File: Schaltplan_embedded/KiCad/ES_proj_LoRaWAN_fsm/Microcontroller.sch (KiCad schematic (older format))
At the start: 15 parts, among them J1 Conn_02x05_Odd_Even, U1 STM32L476RGTx, Y1 Crystal

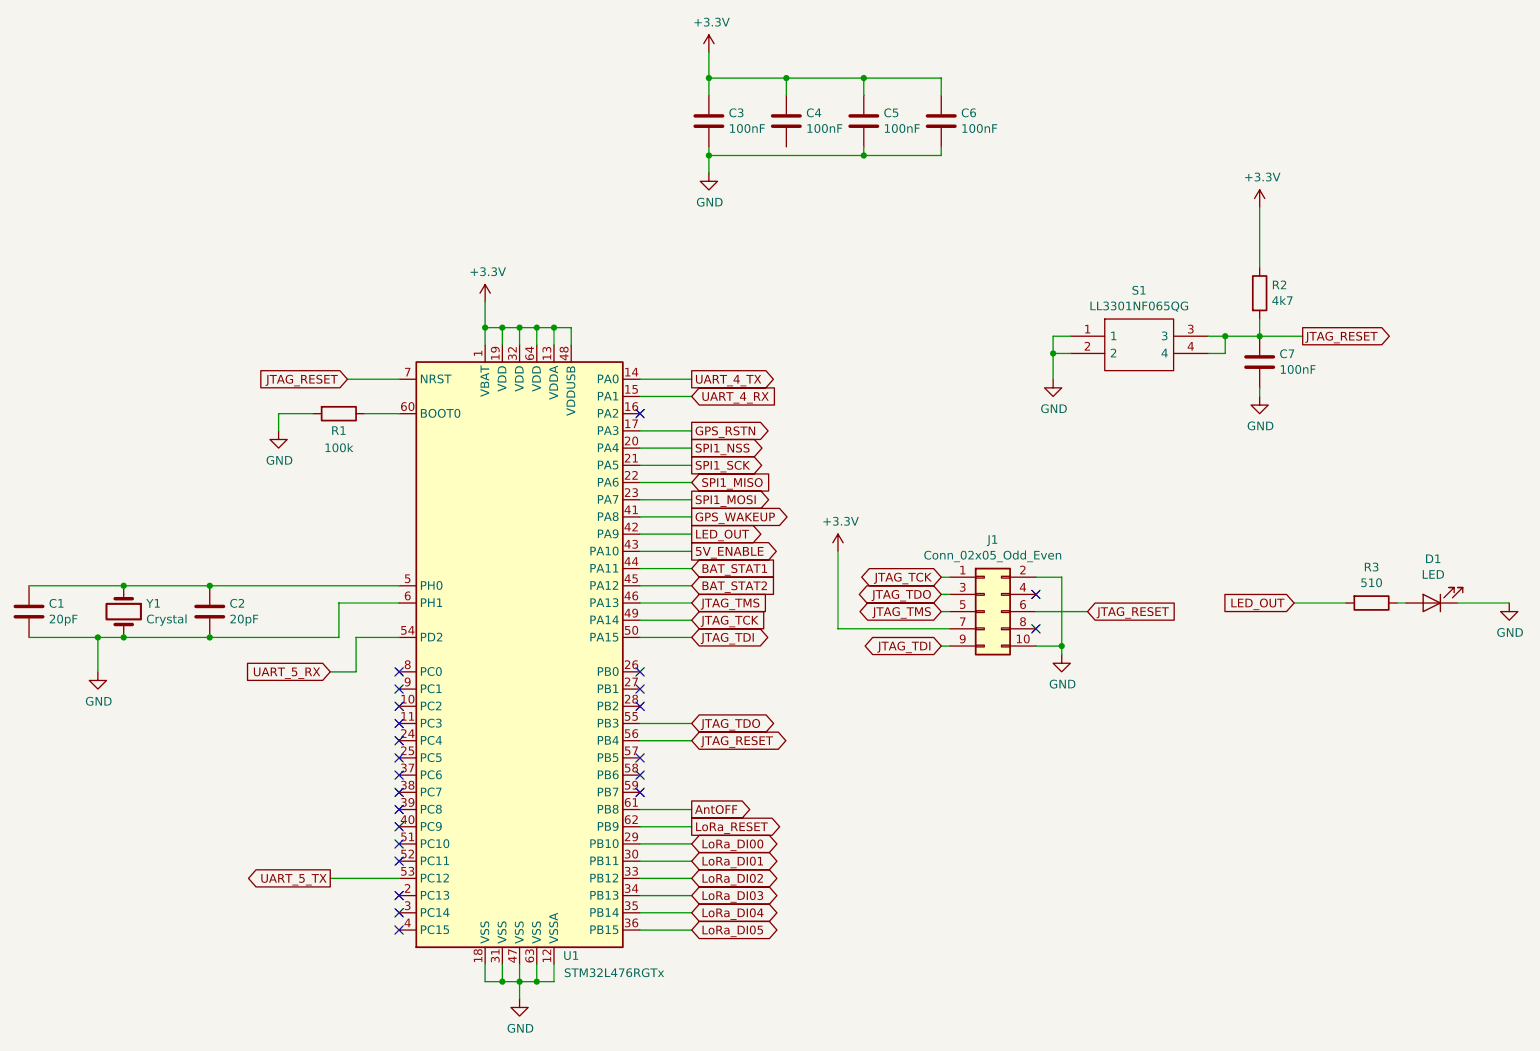
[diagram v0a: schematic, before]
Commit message: no message
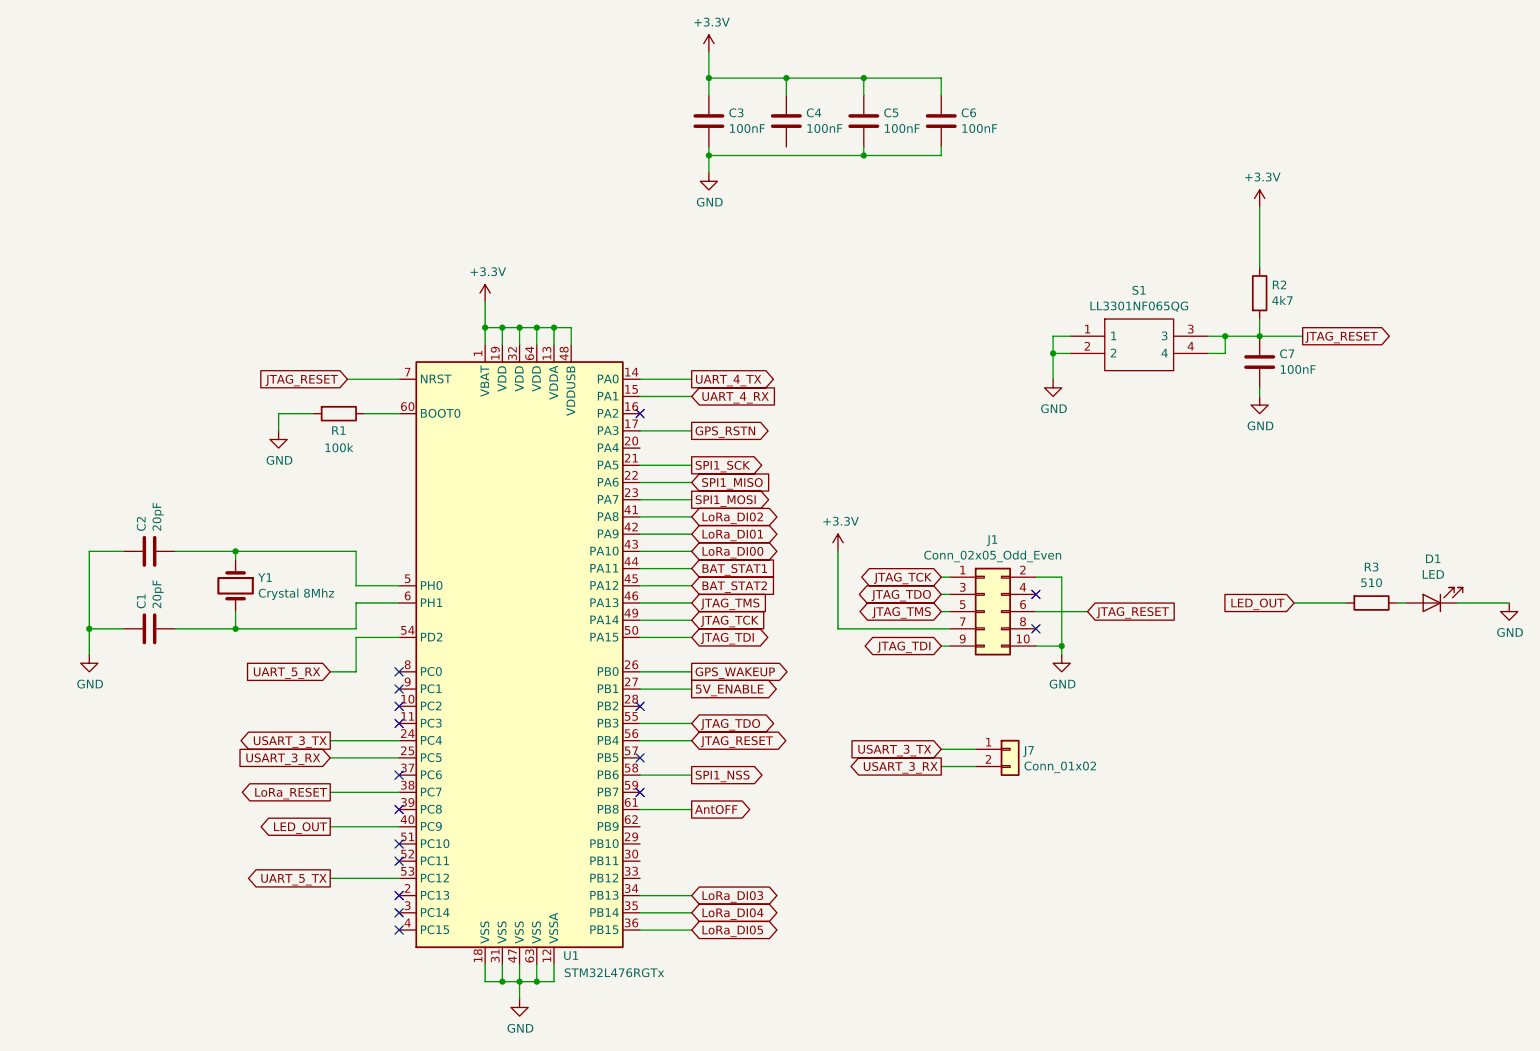
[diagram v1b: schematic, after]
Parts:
- added J7: Conn_01x02, Pin_Headers:Pin_Header_Straight_1x02_Pitch1.00mm, symbol Connector_Generic:Conn_01x02
- Y1: value Crystal -> Crystal 8Mhz; footprint SamacSys_Parts:ABS2532768KHZT -> Crystals:Crystal_SMD_HC49-SD_HandSoldering
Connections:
- net 5V_ENABLE: now also U1.27 (PB1); no longer U1.43 (PA10)
- net GND: now also C1.1, C2.1; no longer C1.2, C2.2, U1.6 (PH1), Y1.2
- net GPS_WAKEUP: now also U1.26 (PB0); no longer U1.41 (PA8)
- net LED_OUT: now also U1.40 (PC9); no longer U1.42 (PA9)
- net LoRa_DI00: now also U1.43 (PA10); no longer U1.29 (PB10)
- net LoRa_DI01: now also U1.42 (PA9); no longer U1.30 (PB11)
- net LoRa_DI02: now also U1.41 (PA8); no longer U1.33 (PB12)
- net LoRa_RESET: now also U1.38 (PC7); no longer U1.62 (PB9)
- net SPI1_NSS: now also U1.58 (PB6); no longer U1.20 (PA4)
- net USART_3_TX: now reaches U1.24 (PC4)
- net USART_3_TX: now also J7.1 (Pin_1)
- net USART_3_RX: now reaches U1.25 (PC5)
- net USART_3_RX: now also J7.2 (Pin_2)
- net at U1.5 (PH0), Y1.1: now also C2.2; no longer C1.1, C2.1
- new net: C1.2, U1.6 (PH1), Y1.2
- no-connect marks 24 -> 17
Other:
- moved on the sheet: C1, C2, Y1
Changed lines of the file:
@@
 L power:GND #PWR0101
 U 1 1 5DC1A6C7
-P 1650 4750
-F 0 "#PWR0101" H 1650 4500 50  0001 C CNN
-F 1 "GND" H 1655 4577 50  0000 C CNN
-F 2 "" H 1650 4750 50  0001 C CNN
-F 3 "" H 1650 4750 50  0001 C CNN
-	1    1650 4750
+P 1600 4650
+F 0 "#PWR0101" H 1600 4400 50  0001 C CNN
+F 1 "GND" H 1605 4477 50  0000 C CNN
+F 2 "" H 1600 4650 50  0001 C CNN
+F 3 "" H 1600 4650 50  0001 C CNN
+	1    1600 4650
 	1    0    0    -1
 $EndComp
@@
 L Device:Crystal Y1
 U 1 1 5DC1A7A3
-P 1800 4400
-F 0 "Y1" V 1754 4531 50  0000 L CNN
-F 1 "Crystal" V 1845 4531 50  0000 L CNN
-F 2 "SamacSys_Parts:ABS2532768KHZT" H 1800 4400 50  0001 C CNN
-F 3 "~" H 1800 4400 50  0001 C CNN
-	1    1800 4400
+P 2450 4250
+F 0 "Y1" V 2404 4381 50  0000 L CNN
+F 1 "Crystal 8Mhz" V 2495 4381 50  0000 L CNN
+F 2 "Crystals:Crystal_SMD_HC49-SD_HandSoldering" H 2450 4250 50  0001 C CNN
+F 3 "~" H 2450 4250 50  0001 C CNN
+	1    2450 4250
 	0    1    1    0
 $EndComp
@@
 L Device:C C1
 U 1 1 5DC1A815
-P 1250 4400
-F 0 "C1" H 1365 4446 50  0000 L CNN
-F 1 "20pF" H 1365 4355 50  0000 L CNN
-F 2 "Capacitors_SMD:C_0603_HandSoldering" H 1288 4250 50  0001 C CNN
-F 3 "~" H 1250 4400 50  0001 C CNN
-	1    1250 4400
-	1    0    0    -1
-$EndComp
-$Comp
-L Device:C C2
-U 1 1 5DC1A899
-P 2300 4400
-F 0 "C2" H 2415 4446 50  0000 L CNN
-F 1 "20pF" H 2415 4355 50  0000 L CNN
-F 2 "Capacitors_SMD:C_0603_HandSoldering" H 2338 4250 50  0001 C CNN
-F 3 "~" H 2300 4400 50  0001 C CNN
-	1    2300 4400
-	1    0    0    -1
-$EndComp
-Wire Wire Line
-	1250 4550 1650 4550
-Wire Wire Line
-	2300 4550 1800 4550
-Connection ~ 1800 4550
-Wire Wire Line
-	1650 4750 1650 4550
-Connection ~ 1650 4550
-Wire Wire Line
-	1650 4550 1800 4550
-Wire Wire Line
-	1250 4250 1800 4250
-Wire Wire Line
-	2300 4250 1800 4250
-Connection ~ 1800 4250
-Connection ~ 2300 4250
-Connection ~ 2300 4550
-Wire Wire Line
-	2300 4550 3050 4550
-Wire Wire Line
-	2300 4250 3400 4250
-Wire Wire Line
-	3050 4550 3050 4350
-Wire Wire Line
-	3050 4350 3400 4350
+P 1950 4500
+F 0 "C1" H 2065 4546 50  0000 L CNN
+F 1 "20pF" H 2065 4455 50  0000 L CNN
+F 2 "Capacitors_SMD:C_0603_HandSoldering" H 1988 4350 50  0001 C CNN
+F 3 "~" H 1950 4500 50  0001 C CNN
+	1    1950 4500
+	0    -1   -1   0
+$EndComp
 $Comp
 L power:GND #PWR0102
@@
 Wire Wire Line
 	6550 1300 6550 1400
-Text GLabel 5100 3450 2    50   Output ~ 0
+Text GLabel 5100 5350 2    50   Output ~ 0
 SPI1_NSS
-Wire Wire Line
-	4800 3450 5100 3450
 Text GLabel 5100 3550 2    50   Output ~ 0
 SPI1_SCK
@@
 Wire Wire Line
 	4800 3650 5100 3650
-Wire Wire Line
-	4800 3750 5100 3750
 Text GLabel 5100 3150 2    50   Input ~ 0
 UART_4_RX
@@
 Wire Wire Line
 	2700 3250 2700 3350
-Text GLabel 5100 3950 2    50   Output ~ 0
+Text GLabel 3000 5650 0    50   Output ~ 0
 LED_OUT
-Wire Wire Line
-	5100 3950 4800 3950
 Text GLabel 8600 4350 0    50   Input ~ 0
 LED_OUT
@@
 Wire Wire Line
 	9550 4350 9850 4350
-Text GLabel 5100 4050 2    51   Output ~ 0
+Text GLabel 5100 4850 2    51   Output ~ 0
 5V_ENABLE
 NoConn ~ 4800 5450
-NoConn ~ 4800 5350
 NoConn ~ 4800 5250
 NoConn ~ 3400 6250
@@
 NoConn ~ 3400 5850
 NoConn ~ 3400 5750
-NoConn ~ 3400 5650
 NoConn ~ 3400 5550
-NoConn ~ 3400 5450
 NoConn ~ 3400 5350
-NoConn ~ 3400 5250
-NoConn ~ 3400 5150
 NoConn ~ 3400 5050
 NoConn ~ 3400 4950
@@
 NoConn ~ 3400 4750
 NoConn ~ 4800 4950
-NoConn ~ 4800 4850
-NoConn ~ 4800 4750
 NoConn ~ 4800 3250
 Text GLabel 3100 3050 0    50   Input ~ 0
@@
 Wire Wire Line
 	4800 4250 5100 4250
-Text GLabel 5100 3850 2    50   Output ~ 0
+Text GLabel 5100 4750 2    50   Output ~ 0
 GPS_WAKEUP
 Text GLabel 5100 3350 2    50   Output ~ 0
@@
 Wire Wire Line
 	4800 3350 5100 3350
-Text GLabel 5100 5850 2    50   BiDi ~ 0
+Text GLabel 5100 3950 2    50   BiDi ~ 0
 LoRa_DI01
-Text GLabel 5100 5750 2    50   BiDi ~ 0
+Text GLabel 5100 4050 2    50   BiDi ~ 0
 LoRa_DI00
-Text GLabel 5100 5950 2    50   BiDi ~ 0
+Text GLabel 5100 3850 2    50   BiDi ~ 0
 LoRa_DI02
 Text GLabel 5100 6050 2    50   BiDi ~ 0
@@
 LoRa_DI05
 Wire Wire Line
-	4800 5750 5100 5750
-Wire Wire Line
-	4800 5850 5100 5850
-Wire Wire Line
-	4800 5950 5100 5950
-Wire Wire Line
 	4800 6050 5100 6050
 Wire Wire Line
@@
 Wire Wire Line
 	4800 6250 5100 6250
-Text GLabel 5100 5650 2    50   Output ~ 0
+Text GLabel 3000 5450 0    50   Output ~ 0
 LoRa_RESET
-Wire Wire Line
-	4800 5650 5100 5650
-$Comp
-L MCU_ST_STM32L4:STM32L476RGTx U1
-U 1 1 5DC1A60F
-P 4100 4650
-F 0 "U1" H 4400 2900 50  0000 C CNN
-F 1 "STM32L476RGTx" H 4650 2800 50  0000 C CNN
-F 2 "Housings_QFP:LQFP-64_10x10mm_Pitch0.5mm" H 3500 2950 50  0001 R CNN
-F 3 "http://www.st.com/st-web-ui/static/active/en/resource/technical/document/datasheet/DM00108832.pdf" H 4100 4650 50  0001 C CNN
-	1    4100 4650
-	1    0    0    -1
-$EndComp
 Wire Wire Line
 	3900 6450 3900 6550
@@
 Wire Wire Line
 	4800 5550 5100 5550
-Wire Wire Line
-	4800 4050 5100 4050
-Wire Wire Line
-	4800 3850 5100 3850
 $Comp
 L power:+3.3V #PWR0114
@@
 Wire Wire Line
 	8200 2800 8400 2800
+Wire Wire Line
+	4800 3750 5100 3750
+Wire Wire Line
+	4800 5350 5100 5350
+Wire Wire Line
+	4800 4050 5100 4050
+Wire Wire Line
+	4800 3950 5100 3950
+Wire Wire Line
+	4800 3850 5100 3850
+Wire Wire Line
+	3000 5650 3400 5650
+$Comp
+L MCU_ST_STM32L4:STM32L476RGTx U1
+U 1 1 5DC1A60F
+P 4100 4650
+F 0 "U1" H 4400 2900 50  0000 C CNN
+F 1 "STM32L476RGTx" H 4650 2800 50  0000 C CNN
+F 2 "Housings_QFP:LQFP-64_10x10mm_Pitch0.5mm" H 3500 2950 50  0001 R CNN
+F 3 "http://www.st.com/st-web-ui/static/active/en/resource/technical/document/datasheet/DM00108832.pdf" H 4100 4650 50  0001 C CNN
+	1    4100 4650
+	1    0    0    -1
+$EndComp
+Wire Wire Line
+	3400 5450 3000 5450
+Wire Wire Line
+	4800 4750 5100 4750
+Wire Wire Line
+	4800 4850 5100 4850
+Text GLabel 3000 5150 0    50   Output ~ 0
+USART_3_TX
+Text GLabel 3000 5250 0    50   Input ~ 0
+USART_3_RX
+Wire Wire Line
+	3000 5250 3400 5250
+Wire Wire Line
+	3000 5150 3400 5150
+$Comp
+L Connector_Generic:Conn_01x02 J7
+U 1 1 5DE2967D
+P 6950 5200
+F 0 "J7" H 7030 5192 50  0000 L CNN
+F 1 "Conn_01x02" H 7030 5101 50  0000 L CNN
+F 2 "Pin_Headers:Pin_Header_Straight_1x02_Pitch1.00mm" H 6950 5200 50  0001 C CNN
+F 3 "~" H 6950 5200 50  0001 C CNN
+	1    6950 5200
+	1    0    0    -1
+$EndComp
+Text GLabel 6550 5200 0    50   Input ~ 0
+USART_3_TX
+Text GLabel 6550 5300 0    50   Output ~ 0
+USART_3_RX
+Wire Wire Line
+	6550 5200 6750 5200
+Wire Wire Line
+	6550 5300 6750 5300
+$Comp
+L Device:C C2
+U 1 1 5DC1A899
+P 1950 4050
+F 0 "C2" H 2065 4096 50  0000 L CNN
+F 1 "20pF" H 2065 4005 50  0000 L CNN
+F 2 "Capacitors_SMD:C_0603_HandSoldering" H 1988 3900 50  0001 C CNN
+F 3 "~" H 1950 4050 50  0001 C CNN
+	1    1950 4050
+	0    -1   -1   0
+$EndComp
+Wire Wire Line
+	3400 4250 3150 4250
+Wire Wire Line
+	3150 4250 3150 4050
+Wire Wire Line
+	3150 4050 2450 4050
+Wire Wire Line
+	2450 4050 2450 4100
+Wire Wire Line
+	3400 4350 3150 4350
+Wire Wire Line
+	3150 4350 3150 4500
+Wire Wire Line
+	3150 4500 2450 4500
+Wire Wire Line
+	2450 4500 2450 4400
+Wire Wire Line
+	1600 4650 1600 4500
+Wire Wire Line
+	1600 4050 1800 4050
+Wire Wire Line
+	1600 4500 1800 4500
+Connection ~ 1600 4500
+Wire Wire Line
+	1600 4500 1600 4050
+Wire Wire Line
+	2100 4050 2450 4050
+Connection ~ 2450 4050
+Connection ~ 2450 4500
+Wire Wire Line
+	2100 4500 2450 4500
 $EndSCHEMATC
